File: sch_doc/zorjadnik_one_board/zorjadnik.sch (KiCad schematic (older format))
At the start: 50 parts, among them J1 OUT1, J10 output GND, J11 power supply GND, J12 spare port, J2 OUT2, J3 Vsb, J4 GND, J6 firmware, J7 cooling fan, J9 power supply Vout, Q1 BCR512, Q2 BCR108, Q3 BCR108, U1 AP1117-33, U2 STM32F030F4Px

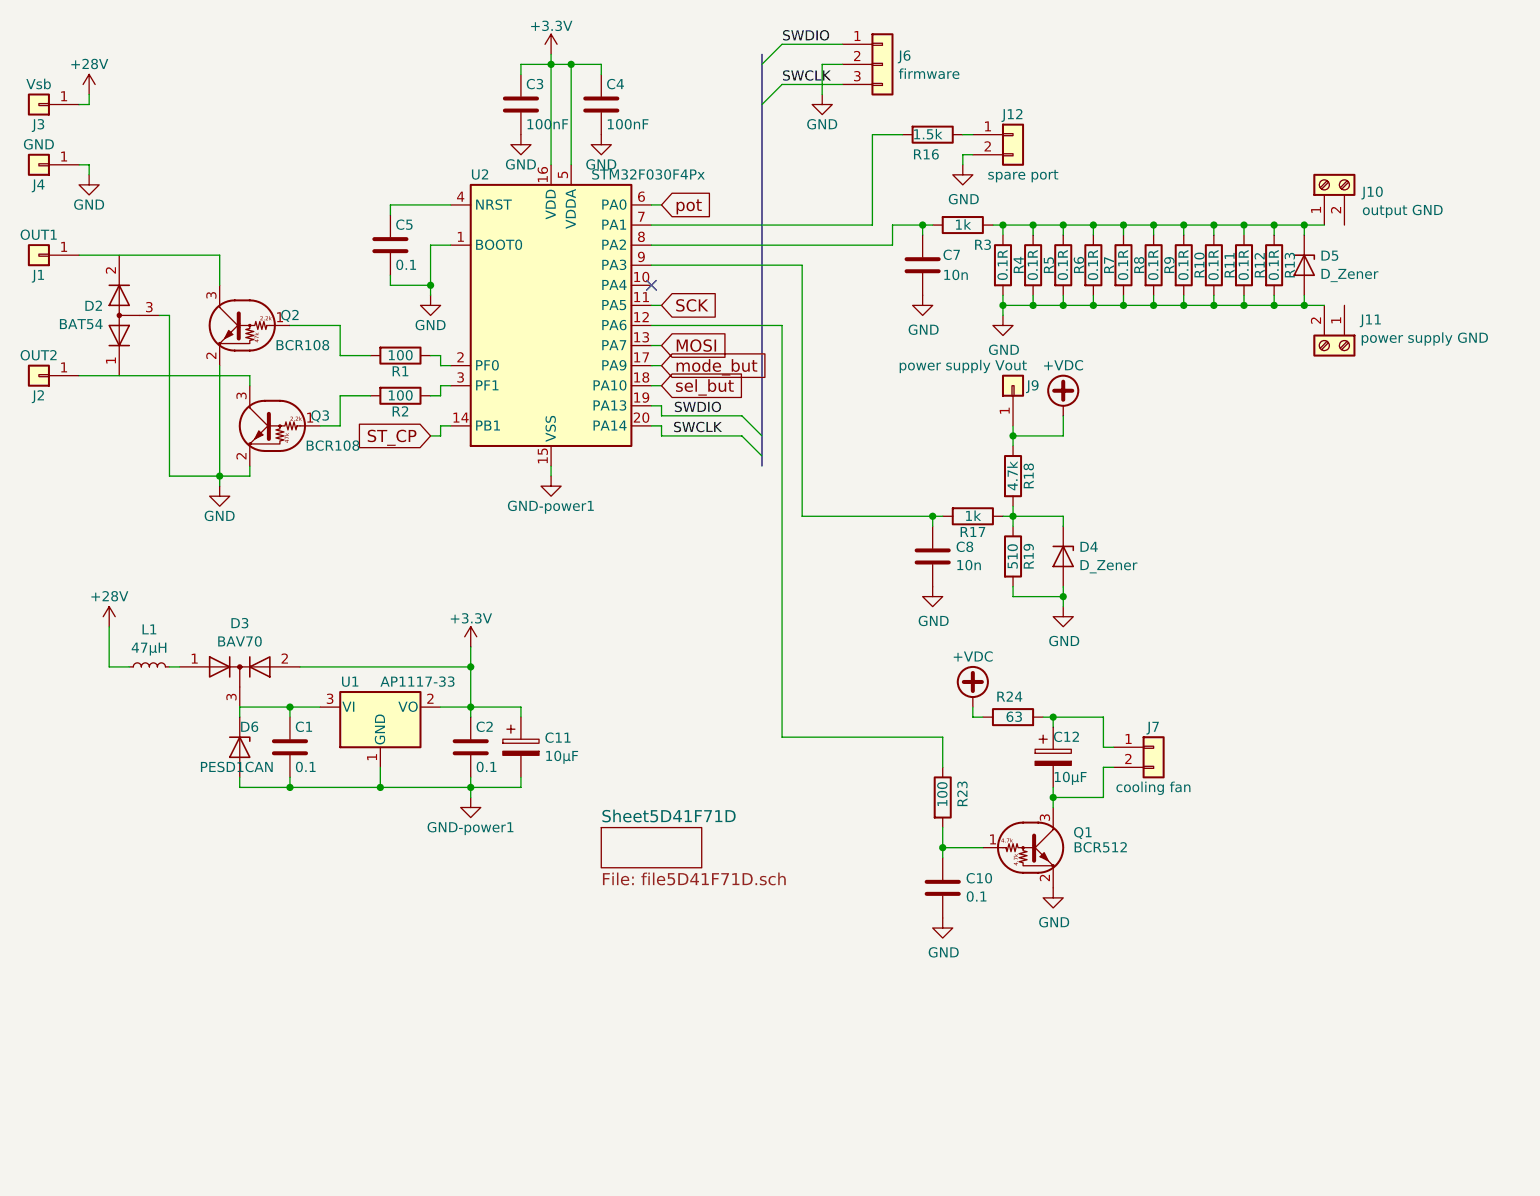
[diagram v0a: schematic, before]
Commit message: добавил сохрааниение настроек, подправил переменник, не проверял
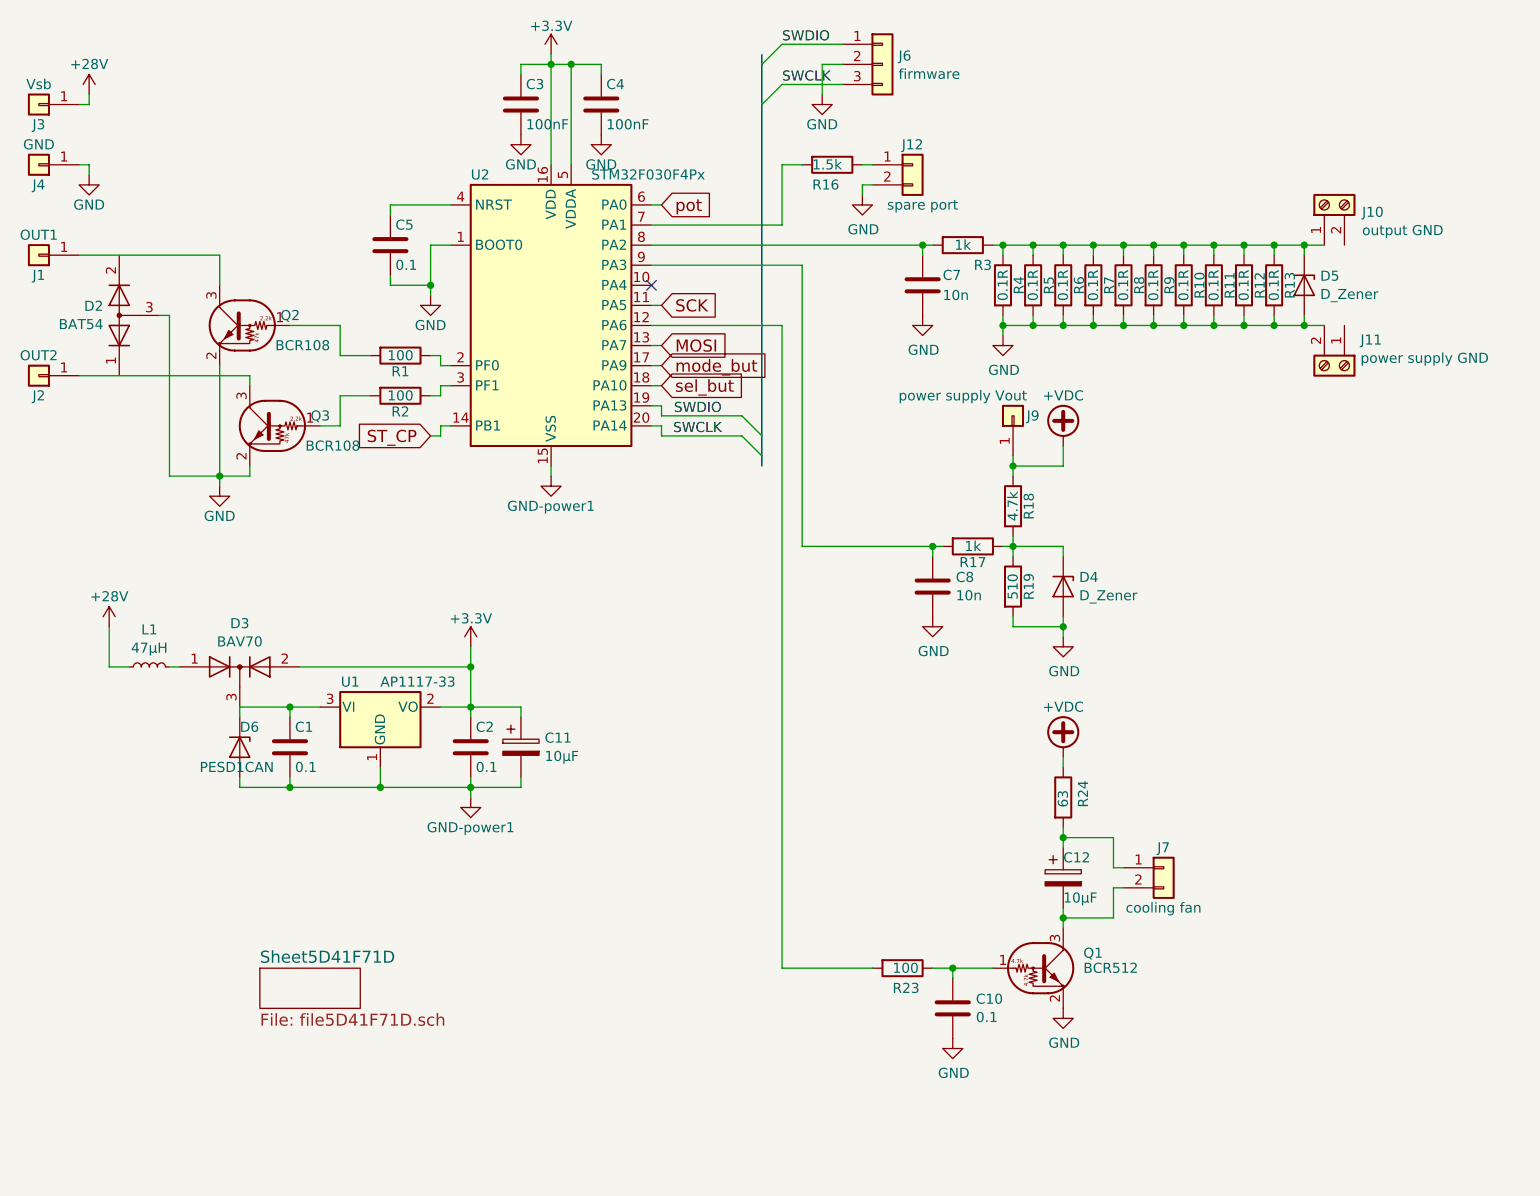
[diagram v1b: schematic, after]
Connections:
- net at U2.12 (PA6): now also R23.2; no longer R23.1
- net at C10.1, Q1.1 (B): now also R23.1; no longer R23.2
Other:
- moved on the sheet: C10, C12, C7, C8, D4, D5, J10, J11, J12, J7, J9, Q1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

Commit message: наладил, как сделаю трансформатор, так будет релиз
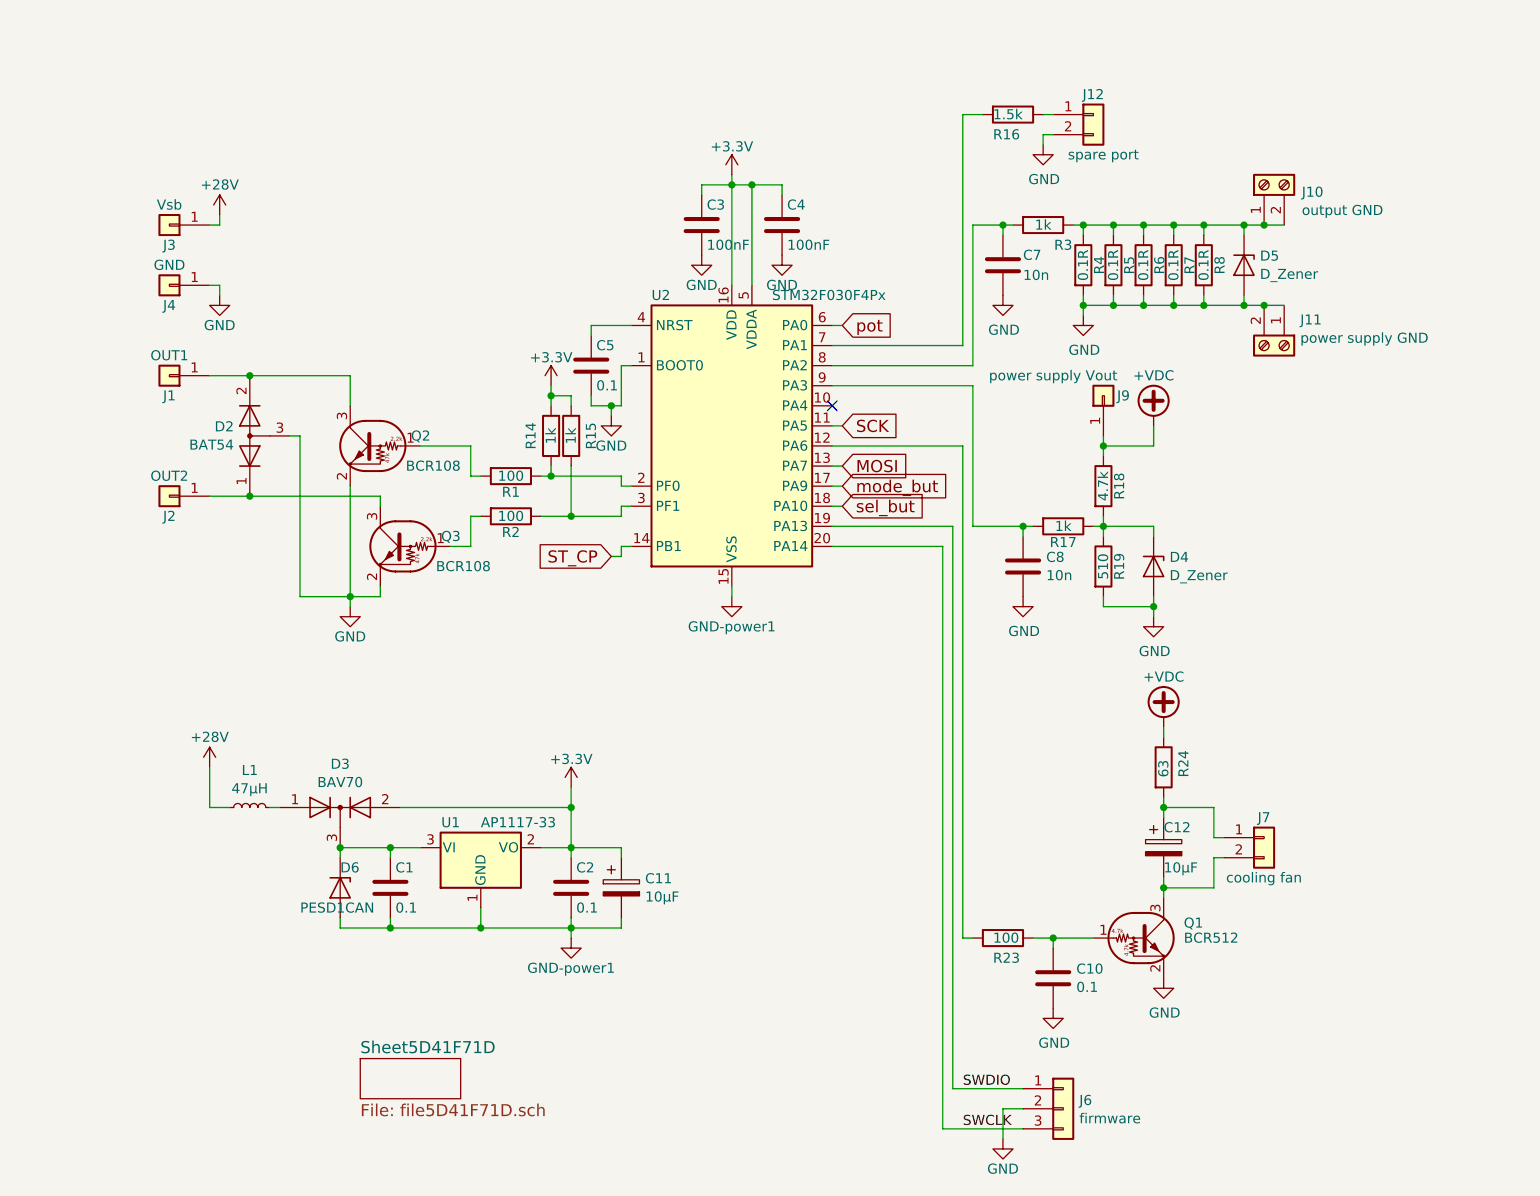
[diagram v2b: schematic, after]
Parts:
- removed R10, R11, R12, R13, R9: 0.1R, Resistor_SMD:R_2010_5025Metric, symbol zorjadnik:R-zorjadnik
- added R14, R15: 1k, Resistor_SMD:R_0805_2012Metric, symbol device:R
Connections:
- net +3V3: now also R14.2, R15.2
- net GND: now also J11.1 (Pin_1)
- net at R1.1, U2.2 (PF0): now also R14.1
- net at R2.1, U2.3 (PF1): now also R15.1
- net at D5.3 (K), J10.1 (Pin_1), R3.1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: now also J10.2 (Pin_2)
- net at J2.1 (Pin_1), Q3.3 (C): now also D2.1 (K)
- net at J1.1 (Pin_1), Q2.3 (C): now also D2.2 (K)
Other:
- moved on the sheet: C1, C10, C11, C12, C2, C3, C4, C5, C7, C8, D2, D3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
